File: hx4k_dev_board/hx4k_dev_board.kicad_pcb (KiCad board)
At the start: 4 copper layers, 85 x 54 mm, 111 parts, among them J1 USB_B, J2 RB1-125B8G1A, J3 Conn_01x08, J4 Conn_02x06_Odd_Even, J5 Conn_02x06_Odd_Even, SW1 SW_SPST, SW2 SW_SPST, SW3 SW_SPST, U1 W9812G6KH-6, U2 CH340E, U3 TPS7A7001DDA, U4 TPS7A7001DDA, U5 RTL8211EG-VB-CG, U6 ICE40HX4K-TQ144, U7 W25Q128JVS, X1 SG-7050CAN, X2 SG-7050CAN

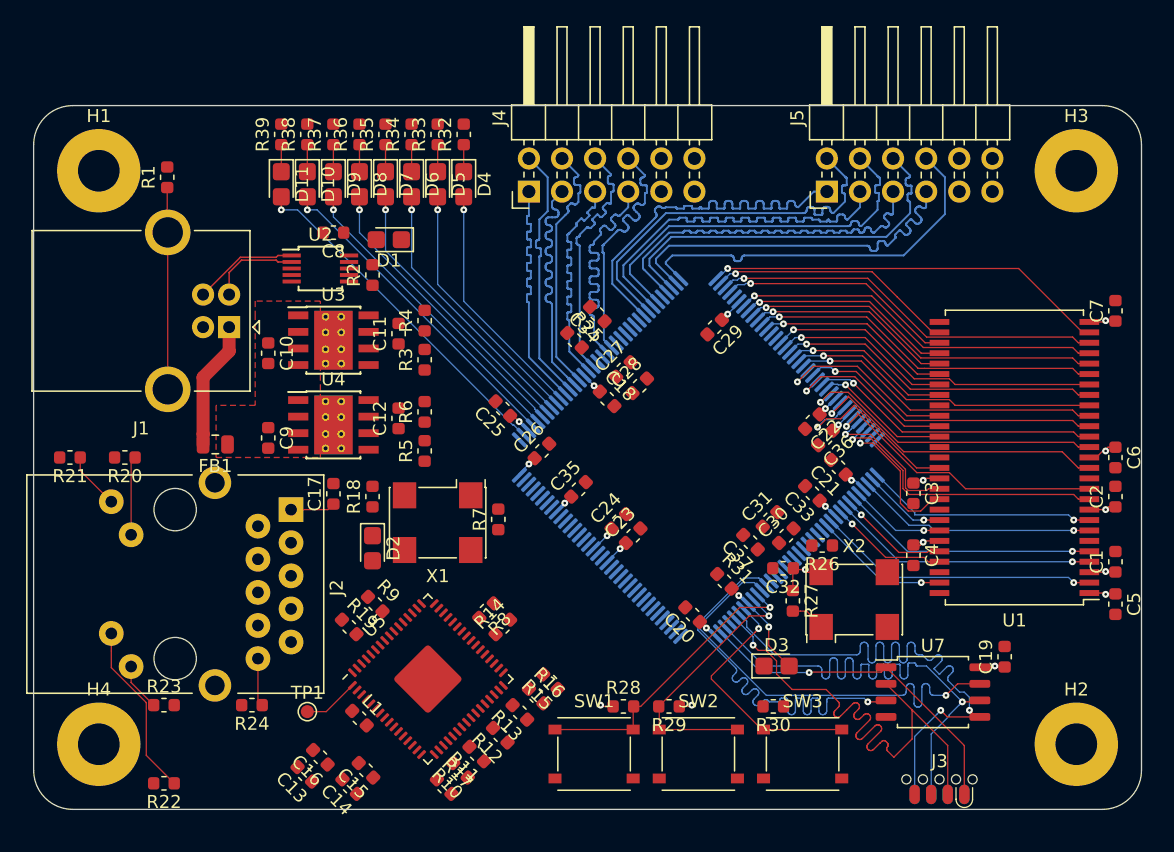
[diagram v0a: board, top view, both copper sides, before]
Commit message: Fully routed
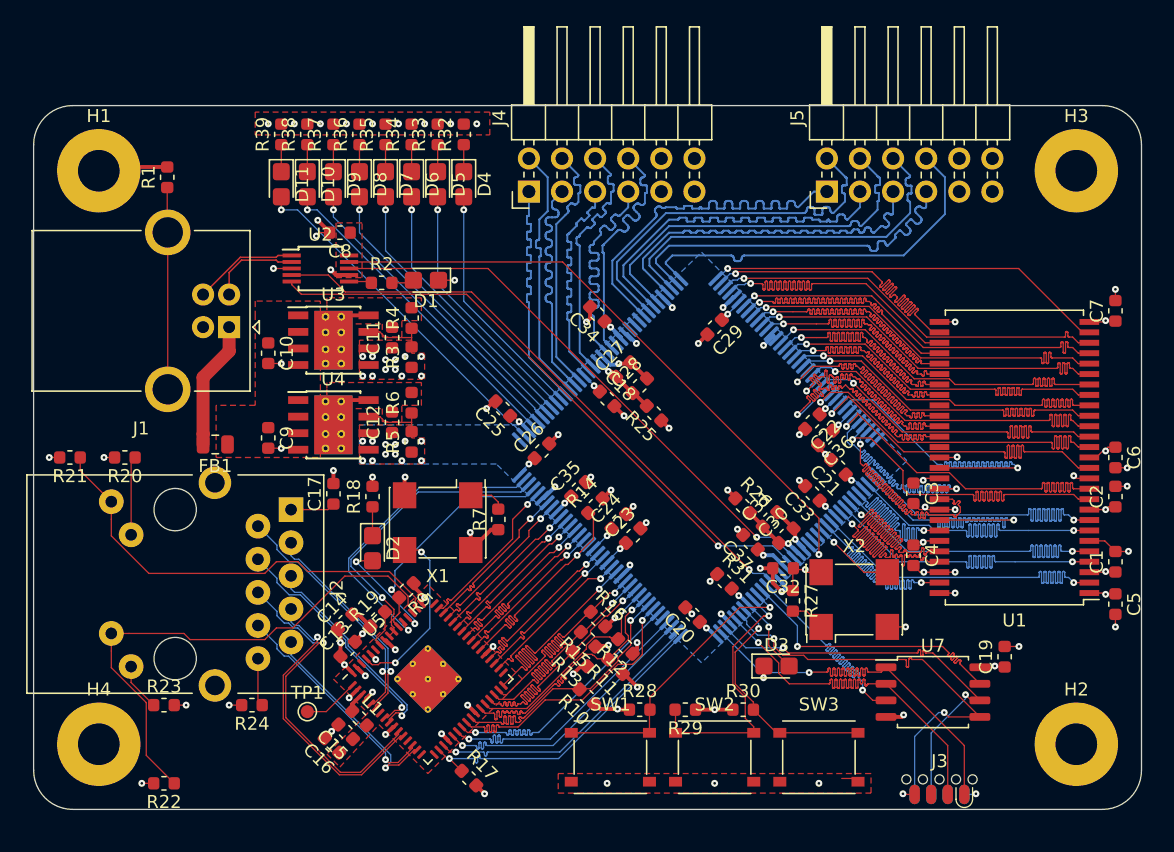
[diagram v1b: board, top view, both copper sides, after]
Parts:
- removed R8: 10k, Resistor_SMD:R_0603_1608Metric
- U5: footprint Package_DFN_QFN:QFN-64-1EP_9x9mm_P0.5mm_EP3.8x3.8mm -> Package_DFN_QFN:QFN-64-1EP_9x9mm_P0.5mm_EP3.8x3.8mm_ThermalVias
- moved C14 12.7 mm to (316.9, 84.6), turned to 45 degrees
- moved R11 12.6 mm to (337.6, 88.0)
- moved R12 11.8 mm to (338.4, 86.5)
- moved R14 11.7 mm to (336.1, 75.7)
- moved R10 11.2 mm to (335.4, 90.3)
- moved C13 10.2 mm to (317.1, 86.7), turned to 45 degrees
- moved R25 8.28 mm to (340.6, 68.6), turned to 135 degrees
- moved R16 7.58 mm to (336.3, 84.4)
- moved R26 6.82 mm to (347.4, 75.7), turned to 315 degrees
- moved R13 6.16 mm to (334.9, 87.5)
- moved R15 4.36 mm to (335.5, 85.9)
- moved D1 4.22 mm to (323.1, 58.4)
- moved C15 3.34 mm to (316.9, 93.0)
- moved R9 2.61 mm to (321.6, 82.2), turned to 225 degrees
- moved R30 2.33 mm to (347.4, 91.3), turned to 0 degrees
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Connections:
- net /POWER/1V8FB renamed /POWER/1V2FB
- net Net-(C27-Pad1) renamed /FPGA/VCCPLL1
- net Net-(C27-Pad2) renamed /FPGA/GNDPLL1
- net Net-(C30-Pad1) renamed /FPGA/VCCPLL0
- net Net-(C30-Pad2) renamed /FPGA/GNDPLL0
- U6 pad 101: /ETHERNET/COL -> /FPGA/ETH_TXD6
- U6 pad 102: /ETHERNET/CS -> /FPGA/ETH_TXD7
- U6 pad 104: /FPGA/ETH_MDC -> /FPGA/ETH_TXER
- U6 pad 107: /FPGA/~ETH_PHYRST -> /FPGA/ETH_MDC
- U6 pad 73: /FPGA/ETH_GTXCLK -> /FPGA/ETH_RXDV
- U6 pad 74: /FPGA/ETH_TXCLK -> /FPGA/ETH_RXD0
- U6 pad 75: /FPGA/ETH_TXD0 -> /FPGA/ETH_RXD1
- U6 pad 76: /FPGA/ETH_TXD1 -> /FPGA/ETH_RXD2
- U6 pad 78: /FPGA/ETH_TXD2 -> /FPGA/ETH_RXD3
- U6 pad 79: /FPGA/ETH_TXD3 -> /ETHERNET/RXCLK
- U6 pad 80: /FPGA/ETH_TXD4 -> /FPGA/ETH_RXD4
- U6 pad 81: /FPGA/ETH_TXD5 -> /FPGA/ETH_RXD5
- U6 pad 82: /FPGA/ETH_TXD6 -> /FPGA/ETH_RXD6
- U6 pad 83: /FPGA/ETH_TXD7 -> /FPGA/ETH_RXD7
- U6 pad 84: /FPGA/ETH_TXEN -> /FPGA/ETH_RXER
- U6 pad 85: /FPGA/ETH_TXER -> /ETHERNET/COL
- U6 pad 87: /ETHERNET/RXCLK -> /ETHERNET/CS
- U6 pad 88: /FPGA/ETH_RXD0 -> /FPGA/ETH_GTXCLK
- U6 pad 90: /FPGA/ETH_RXD1 -> /FPGA/ETH_TXEN
- U6 pad 91: /FPGA/ETH_RXD2 -> /FPGA/ETH_TXD0
- U6 pad 93: /FPGA/ETH_RXD3 -> /FPGA/~ETH_PHYRST
- U6 pad 94: /FPGA/ETH_RXD4 -> /FPGA/ETH_TXD1
- U6 pad 95: /FPGA/ETH_RXD5 -> /FPGA/ETH_TXD2
- U6 pad 96: /FPGA/ETH_RXD6 -> /FPGA/ETH_TXD3
- U6 pad 97: /FPGA/ETH_RXD7 -> /FPGA/ETH_TXCLK
- U6 pad 98: /FPGA/ETH_RXDV -> /FPGA/ETH_TXD4
- U6 pad 99: /FPGA/ETH_RXER -> /FPGA/ETH_TXD5
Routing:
- net GND: track 0.00 -> 84.6 mm, vias 0 -> 74
- net /USB_UART/UART_RX: track 0.00 -> 48.1 mm, vias 0 -> 1
- net /FPGA/UART_CTS: track 0.00 -> 47.3 mm, vias 0 -> 1
- net /FPGA/~UART_RTS: track 0.00 -> 46.5 mm, vias 0 -> 1
- net /FPGA/UART_RX: track 0.00 -> 44.2 mm, vias 0 -> 1
- net +3V3: track 37.6 -> 68.7 mm, vias 19 -> 50
- net /ETHERNET/LED_G_HIGH: track 4.38 -> 34.0 mm
- net /ETHERNET/LED_Y_HIGH: track 13.5 -> 40.5 mm
- net /ETHERNET/MDI2_P: track 0.00 -> 25.7 mm, vias 0 -> 1
- net /FPGA/ETH_RXDV: track 0.00 -> 24.9 mm, vias 0 -> 1
- net /SDRAM/DATA11: track 6.41 -> 31.2 mm
- net /FPGA/ETH_MDC: track 0.00 -> 24.2 mm, vias 0 -> 1
- net /SDRAM/DATA12: track 7.36 -> 31.0 mm
- net /FPGA/~ETH_PME_INT: track 0.00 -> 23.6 mm, vias 0 -> 1
- net /ETHERNET/MDI2_N: track 0.00 -> 23.3 mm, vias 0 -> 1
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- added copper zone on B.Cu, net +1V2
- added copper zone on F.Cu, net +1V2
- added copper zone on F.Cu, net +3V3
- added copper zone on In2.Cu, net +3V3
- added copper zone on F.Cu, net /ETHERNET/VDD
- added copper zone on F.Cu, net GND
- added copper zone on In1.Cu, net GND
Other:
- net class Power added: clearance 0.0889, trace_width 0.3, via_dia 0.53, via_drill 0.2
